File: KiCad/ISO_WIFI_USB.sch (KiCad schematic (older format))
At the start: 27 parts, among them P6 CONN_02X03, P7 CONN_02X03, P8 USB_B, SW3 SWITCH_INV, T1 da2303, U19 TLV73333PDBVT, U35 ADUM1402BRWZ, U36 ISO7341c_spi, U40 CP2102N-A01-GQFN24, U5 ESP-12F, U6 SN6505A

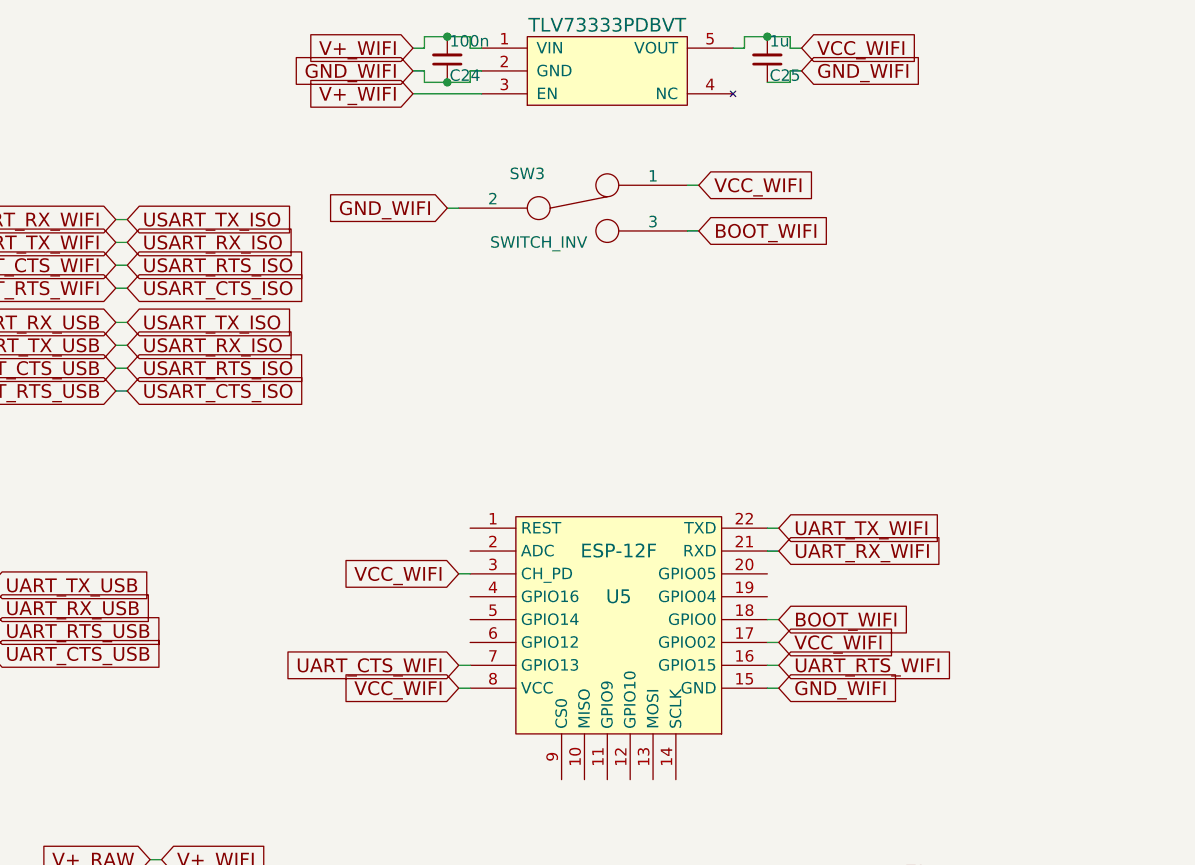
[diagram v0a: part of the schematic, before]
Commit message: kicad
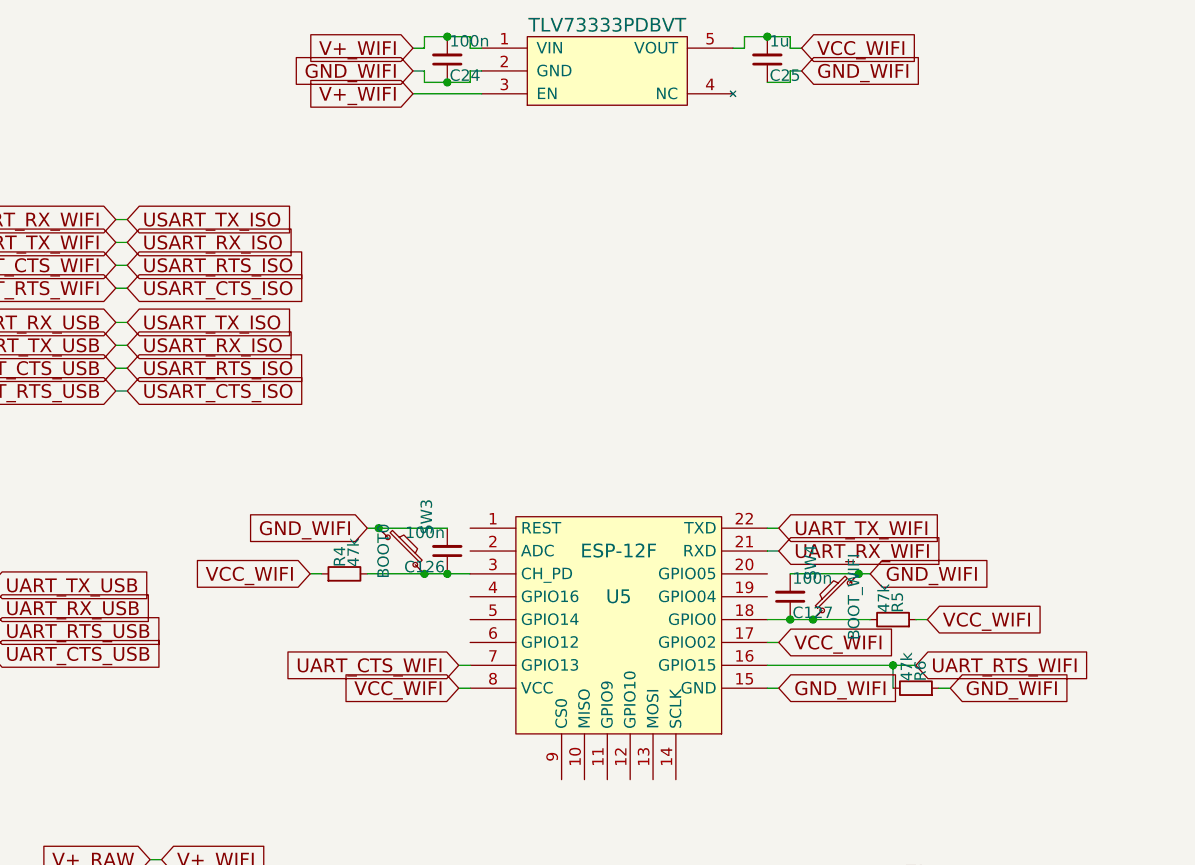
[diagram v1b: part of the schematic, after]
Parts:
- removed SW3: SWITCH_INV, Buttons_Switches_SMD:SW_SPST_B3U-1100P-B, symbol SWITCH_INV
- added C126, C127: 100n, Capacitors_SMD:C_0402, symbol C_Small
- added R4, R5, R6: 47k, Resistors_SMD:R_0402, symbol R_Small
- added SW3: BOOT0, Buttons_Switches_SMD:SW_SPST_B3U-3000P-B, symbol SW_PUSH_SMALL
- added SW4: BOOT_WIFI, Buttons_Switches_SMD:SW_SPST_B3U-1000P, symbol SW_PUSH_SMALL
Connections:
- net GND_ISO_UART: now also C126.2, C127.2, R6.1, SW3.2, SW4.2
- net UART_RTS_USB: now also R6.2
- net VCC_WIFI: now also R4.1, R5.1; no longer U5.3 (CH_PD)
- net BOOT_WIFI: no longer names the net of U5.18 (GPIO0)
- net BOOT_WIFI: now also C127.1, R5.2, SW4.1
- new net: C126.1, R4.2, SW3.1, U5.3 (CH_PD)
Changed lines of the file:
@@
 Text GLabel 7750 3700 2    60   Input ~ 0
 GND_WIFI
-Text GLabel 7750 3600 2    60   Input ~ 0
+Text GLabel 8350 3600 2    60   Input ~ 0
 UART_RTS_WIFI
 Text GLabel 6350 3600 0    60   Input ~ 0
@@
 	6350 3600 6400 3600
 Wire Wire Line
-	7700 3600 7750 3600
+	7700 3600 8350 3600
 Wire Wire Line
 	4250 3350 4300 3350
@@
 Text GLabel 3000 3350 0    60   Input ~ 0
 VIO_USB
-Text GLabel 6350 3200 0    60   Input ~ 0
-VCC_WIFI
-Wire Wire Line
-	6350 3200 6400 3200
 $Comp
 L C_Small C115
@@
 Text GLabel 7750 3500 2    60   Input ~ 0
 VCC_WIFI
-Text GLabel 7750 3400 2    60   Input ~ 0
-BOOT_WIFI
 Wire Wire Line
 	7700 3500 7750 3500
-Wire Wire Line
-	7700 3400 7750 3400
-Text GLabel 7400 1500 2    60   Input ~ 0
+Text GLabel 8400 3400 2    60   Input ~ 0
 VCC_WIFI
-Text GLabel 6300 1600 0    60   Input ~ 0
+Text GLabel 8150 3200 2    60   Input ~ 0
 GND_WIFI
-Text GLabel 7400 1700 2    60   Input ~ 0
-BOOT_WIFI
-$Comp
-L SWITCH_INV SW3
-U 1 1 58E05F38
-P 6850 1600
-F 0 "SW3" H 6650 1750 50  0000 C CNN
-F 1 "SWITCH_INV" H 6700 1450 50  0000 C CNN
-F 2 "Buttons_Switches_SMD:SW_SPST_B3U-1100P-B" H 6850 1600 50  0001 C CNN
-F 3 "" H 6850 1600 50  0000 C CNN
-	1    6850 1600
-	1    0    0    -1
-$EndComp
-Wire Wire Line
-	6300 1600 6350 1600
-Wire Wire Line
-	7350 1500 7400 1500
-Wire Wire Line
-	7350 1700 7400 1700
 Wire Wire Line
 	9150 5400 9050 5400
@@
 	1    0    0    -1
 $EndComp
+$Comp
+L R_Small R5
+U 1 1 58E54546
+P 8250 3400
+F 0 "R5" H 8280 3420 50  0000 L CNN
+F 1 "47k" H 8280 3360 50  0000 L CNN
+F 2 "Resistors_SMD:R_0402" H 8250 3400 50  0001 C CNN
+F 3 "" H 8250 3400 50  0000 C CNN
+F 4 "RC0402FR-0747KL" H 8250 3400 60  0001 C CNN "manf#"
+	1    8250 3400
+	0    1    -1   0
+$EndComp
+$Comp
+L SW_PUSH_SMALL SW4
+U 1 1 58E5454F
+P 8000 3300
+F 0 "SW4" H 8150 3410 50  0000 C CNN
+F 1 "BOOT_WIFI" H 8000 3221 50  0000 C CNN
+F 2 "Buttons_Switches_SMD:SW_SPST_B3U-1000P" H 8000 3300 50  0001 C CNN
+F 3 "" H 8000 3300 50  0000 C CNN
+F 4 "B3U3000PMB" H 8000 3300 60  0001 C CNN "manf#"
+	1    8000 3300
+	0    -1   -1   0
+$EndComp
+$Comp
+L C_Small C127
+U 1 1 58E54F0F
+P 7800 3300
+F 0 "C127" H 7810 3370 50  0000 L CNN
+F 1 "100n" H 7810 3220 50  0000 L CNN
+F 2 "Capacitors_SMD:C_0402" H 7800 3300 50  0001 C CNN
+F 3 "" H 7800 3300 50  0000 C CNN
+F 4 "MC0402B104K160CT" H 7800 3300 60  0001 C CNN "manf#"
+	1    7800 3300
+	1    0    0    1
+$EndComp
+Wire Wire Line
+	7700 3400 8150 3400
+Connection ~ 7800 3400
+Connection ~ 7900 3400
+Wire Wire Line
+	8350 3400 8400 3400
+Wire Wire Line
+	7800 3200 8150 3200
+Connection ~ 8100 3200
+Text GLabel 5700 3200 0    60   Input ~ 0
+VCC_WIFI
+Text GLabel 5950 3000 0    60   Input ~ 0
+GND_WIFI
+$Comp
+L R_Small R4
+U 1 1 58E56B55
+P 5850 3200
+F 0 "R4" H 5880 3220 50  0000 L CNN
+F 1 "47k" H 5880 3160 50  0000 L CNN
+F 2 "Resistors_SMD:R_0402" H 5850 3200 50  0001 C CNN
+F 3 "" H 5850 3200 50  0000 C CNN
+F 4 "RC0402FR-0747KL" H 5850 3200 60  0001 C CNN "manf#"
+	1    5850 3200
+	0    -1   -1   0
+$EndComp
+$Comp
+L SW_PUSH_SMALL SW3
+U 1 1 58E56B5C
+P 6100 3100
+F 0 "SW3" H 6250 3210 50  0000 C CNN
+F 1 "BOOT0" H 6100 3021 50  0000 C CNN
+F 2 "Buttons_Switches_SMD:SW_SPST_B3U-3000P-B" H 6100 3100 50  0001 C CNN
+F 3 "" H 6100 3100 50  0000 C CNN
+F 4 "B3U1000P" H 6100 3100 60  0001 C CNN "manf#"
+	1    6100 3100
+	0    1    -1   0
+$EndComp
+$Comp
+L C_Small C126
+U 1 1 58E56B64
+P 6300 3100
+F 0 "C126" H 6310 3170 50  0000 L CNN
+F 1 "100n" H 6310 3020 50  0000 L CNN
+F 2 "Capacitors_SMD:C_0402" H 6300 3100 50  0001 C CNN
+F 3 "" H 6300 3100 50  0000 C CNN
+F 4 "MC0402B104K160CT" H 6300 3100 60  0001 C CNN "manf#"
+	1    6300 3100
+	-1   0    0    1
+$EndComp
+Wire Wire Line
+	6400 3200 5950 3200
+Connection ~ 6300 3200
+Connection ~ 6200 3200
+Wire Wire Line
+	5750 3200 5700 3200
+Wire Wire Line
+	6300 3000 5950 3000
+Connection ~ 6000 3000
+$Comp
+L R_Small R6
+U 1 1 58E572B8
+P 8350 3700
+F 0 "R6" H 8380 3720 50  0000 L CNN
+F 1 "47k" H 8380 3660 50  0000 L CNN
+F 2 "Resistors_SMD:R_0402" H 8350 3700 50  0001 C CNN
+F 3 "" H 8350 3700 50  0000 C CNN
+F 4 "RC0402FR-0747KL" H 8350 3700 60  0001 C CNN "manf#"
+	1    8350 3700
+	0    1    -1   0
+$EndComp
+Text GLabel 8500 3700 2    60   Input ~ 0
+GND_WIFI
+Wire Wire Line
+	8500 3700 8450 3700
+Wire Wire Line
+	8250 3600 8250 3700
+Connection ~ 8250 3600
 $EndSCHEMATC

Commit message: kicad
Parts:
- T1: manf# DA2303 -> DA2303-ALD
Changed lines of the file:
@@
 F 2 "SMT_Power_Transformer:SMT Power Transformer" H 8350 5000 50  0001 C CNN
 F 3 "" H 8350 5000 50  0000 C CNN
-F 4 "DA2303" H 8350 5000 60  0001 C CNN "manf#"
+F 4 "DA2303-ALD" H 8350 5000 60  0001 C CNN "manf#"
 	1    8350 5000
 	1    0    0    -1
